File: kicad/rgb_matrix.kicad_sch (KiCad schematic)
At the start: 75 parts

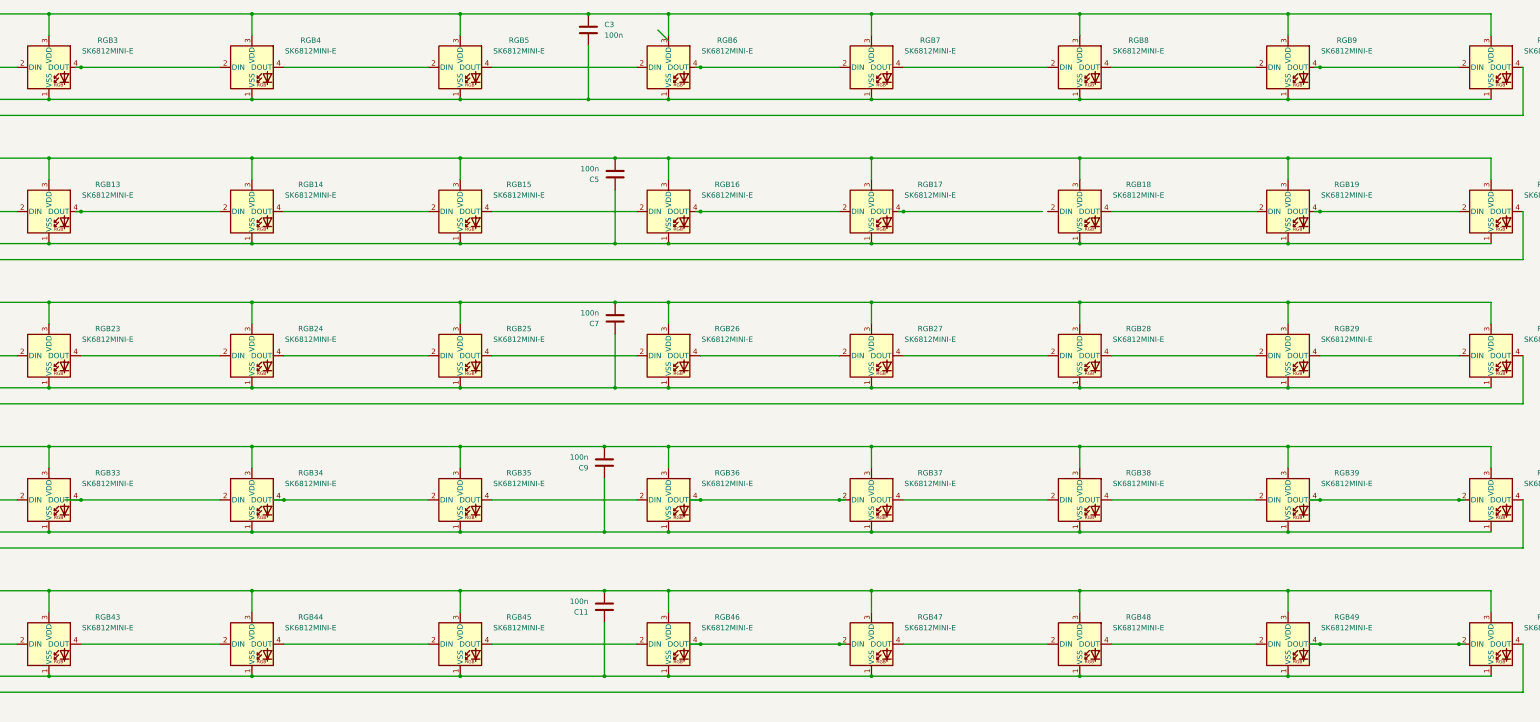
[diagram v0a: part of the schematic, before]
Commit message: pcb done hopefully
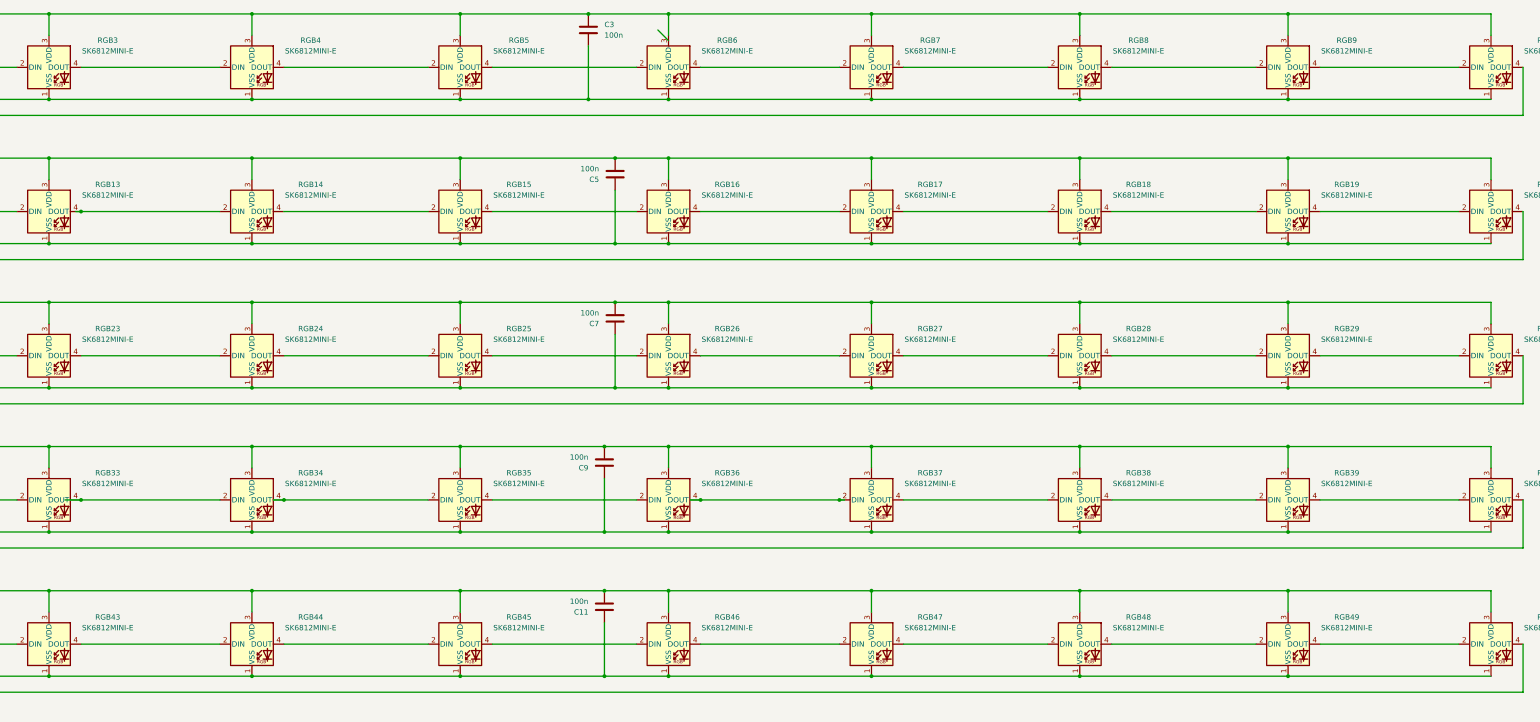
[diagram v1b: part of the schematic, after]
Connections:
- net at RGB18.2 (DIN): now also RGB17.4 (DOUT)
